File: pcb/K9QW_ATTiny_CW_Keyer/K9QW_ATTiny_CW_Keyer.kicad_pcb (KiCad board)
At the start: 2 copper layers, 50.8 x 31.8 mm, 34 parts, among them J1 Power Input, J2 AudioJack4, J3 AudioJack4, J4 Sidetone, J5 Mounting Hole, Q1 AO3401A, Q2 MMBT3904, Q3 MMBT2222A, Q4 MMBT3904, SW1 Power Switch, SW2 Command, U1 ATtiny85-20P, U2 LD1117S33TR_SOT223

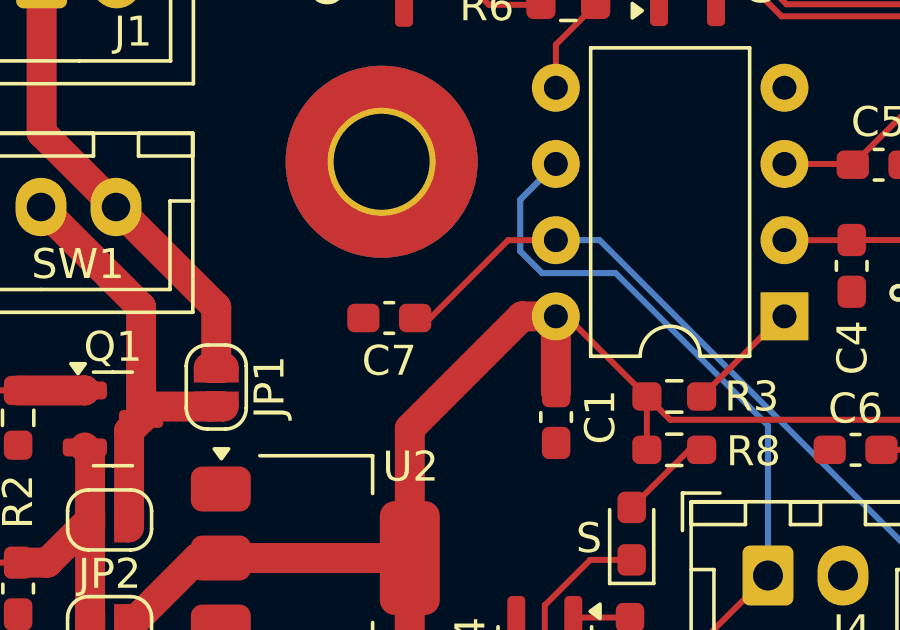
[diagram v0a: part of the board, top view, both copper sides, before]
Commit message: Minor
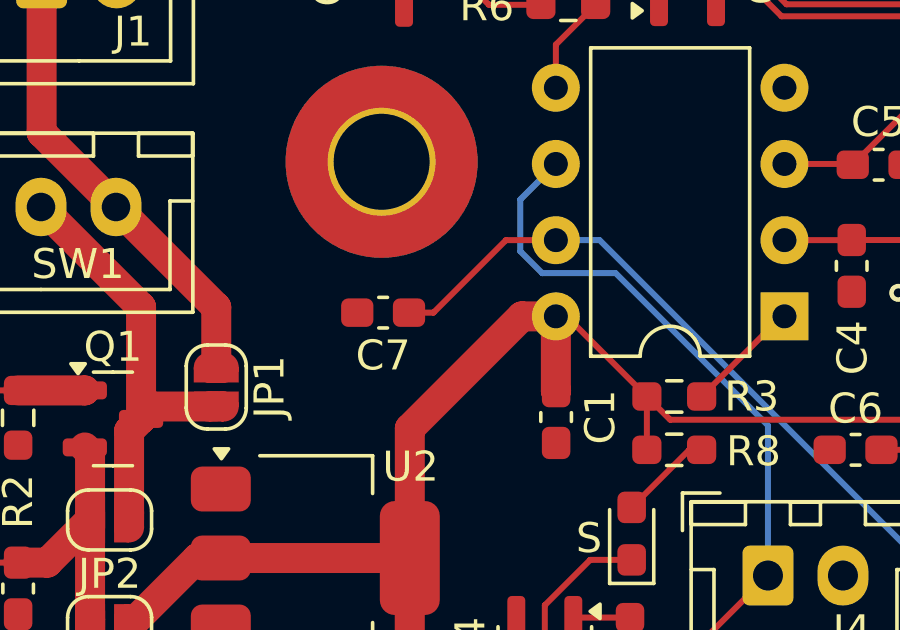
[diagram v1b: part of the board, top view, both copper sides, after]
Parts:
- moved C7 0.27 mm to (145.6, 102.6)
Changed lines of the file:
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@@
 	(footprint "Capacitor_SMD:C_0603_1608Metric_Pad1.08x0.95mm_HandSolder"
 		(layer "F.Cu")
-		(at 145.8468 102.743 180)
+		(at 145.6436 102.5652 180)
 		(descr "Capacitor SMD 0603 (1608 Metric), square (rectangular) end terminal, IPC_7351 nominal with elongated pad for handsoldering. (Body size source: IPC-SM-782 page 76, https://www.pcb-3d.com/wordpress/wp-content/uploads/ipc-sm-782a_amendment_1_and_2.pdf), generated with kicad-footprint-generator")
 		(tags "capacitor handsolder")
@@
 	)
 	(segment
-		(start 147.2184 102.743)
-		(end 149.813 100.1484)
+		(start 151.401 100.1484)
+		(end 149.7368 100.1484)
 		(width 0.2)
 		(layer "F.Cu")
@@
 	)
 	(segment
-		(start 146.7093 102.743)
-		(end 147.2184 102.743)
+		(start 147.32 102.5652)
+		(end 146.7093 102.5652)
 		(width 0.2)
 		(layer "F.Cu")
@@
 	)
 	(segment
-		(start 167.7428 111.161)
-		(end 174.2428 111.161)
+		(start 149.7368 100.1484)
+		(end 147.32 102.5652)
 		(width 0.2)
 		(layer "F.Cu")
@@
 	)
 	(segment
-		(start 149.813 100.1484)
-		(end 151.401 100.1484)
+		(start 167.7428 111.161)
+		(end 174.2428 111.161)
 		(width 0.2)
 		(layer "F.Cu")
